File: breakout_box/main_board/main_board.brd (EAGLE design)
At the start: 60 x 120 mm, 31 parts, among them CN1 19PIN_LEMO, Q1 DMP3099L, Q2 DSS6060

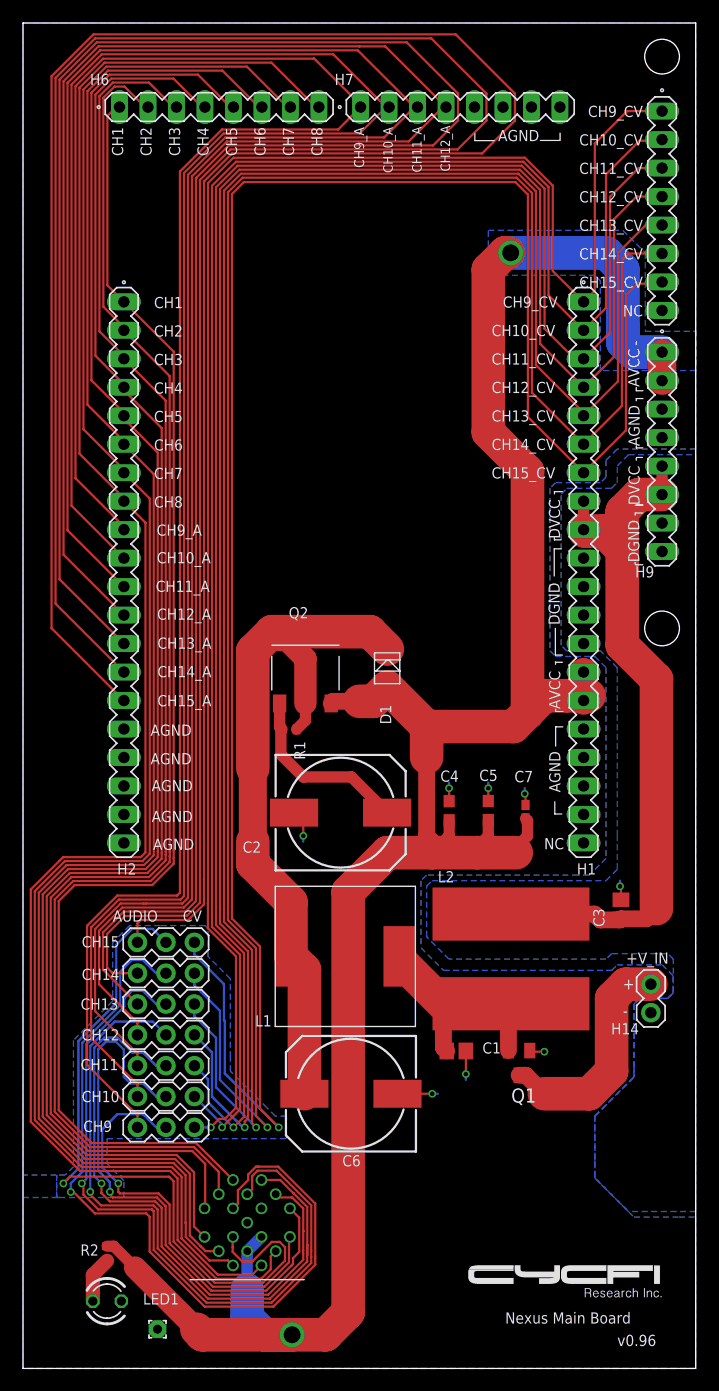
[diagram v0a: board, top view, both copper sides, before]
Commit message: commit and push eagle files for Nexus v2.3
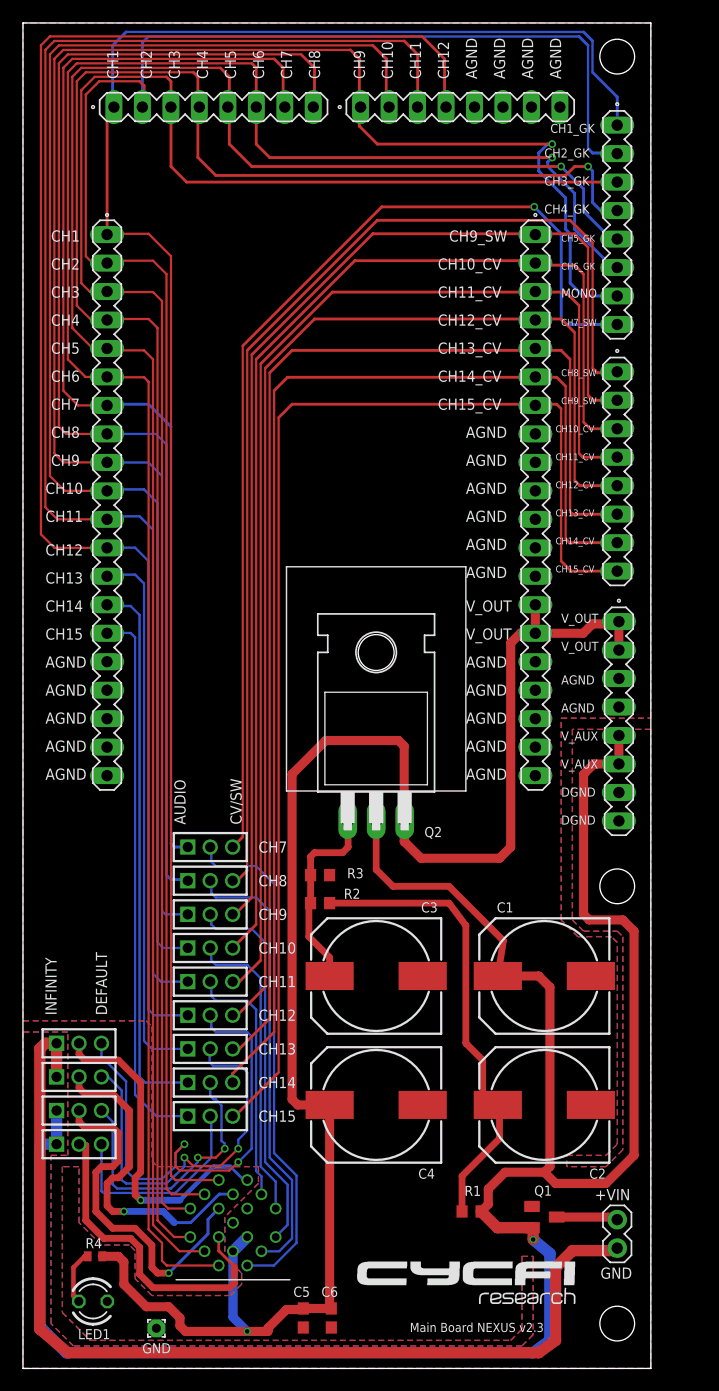
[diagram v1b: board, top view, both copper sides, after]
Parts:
- removed C7: 1nF, resistor:C0402K
- removed D1: FM4004W, CYCFI_diode:SMX
- removed H10, H11, H12, H13, H5: (no value), con-lstb:MA03-1_
- removed H14: MA02-1, con-lstb:MA02-1
- removed H9: (no value), con-lstb:MA08-1
- removed L1: 1mH, inductors:SDR
- removed L2: 82uH, resistor:L1280
- added H17: (no value), con-lstb:MA08-1
- added JP1, JP10, JP11, JP12, JP13, JP2, JP3, JP4, JP5, JP6, JP7, JP8, JP9: (no value), pinhead-2:1X03M
- added R3: 12k, resistor:R0603
- added R4: 4.7k, resistor:R0402
- C1, C3: value 22uF -> 470uF; device resistor:C0805 -> resistor:140CLH-1010
- C4: value 1uF -> 470uF; device resistor:C0603 -> resistor:140CLH-1010
- C5: value 10uF -> 1uF
- C6: value 1000uF -> 0.1uF; device resistor:140CLH-1010 -> resistor:C0603
- H1, H2: value (none) -> DNP
- H3, H4: device con-lstb:MA03-1_ -> con-lstb:MA08-1
- H6: value (none) -> MA02-1; device con-lstb:MA08-1 -> con-lstb:MA02-1
- Q2: value DSS6060 -> TIP122; device CYCFI_semicon:SOT-223-4 -> CYCFI_semicon:TO-220H
- R1: value 1k -> 220R; device resistor:R0402 -> resistor:R0603
- R2: value 4.7k -> 220R; device resistor:R0402 -> resistor:R0603
- moved H6 106.6 mm to (53.0, 12.0), turned to 90 degrees
- moved H4 81.6 mm to (39.0, 112.5)
- moved H3 80.1 mm to (17.0, 112.5)
- moved C5 48.2 mm to (25.0, 4.50), turned to 270 degrees
- moved R1 46.0 mm to (40.0, 14.0)
- moved H8 45.7 mm to (53.1, 57.7)
- moved R2 36.6 mm to (26.5, 41.5), turned to 0 degrees
- moved H7 35.4 mm to (53.0, 80.0), turned to 270 degrees
- moved C2 31.8 mm to (46.5, 23.5), turned to 180 degrees
- moved C4 27.0 mm to (31.5, 23.5), turned to 180 degrees
- moved C3 22.6 mm to (31.5, 35.0), turned to 180 degrees
- moved C6 20.1 mm to (27.5, 4.50), turned to 270 degrees
- moved Q1 13.9 mm to (46.5, 13.5), turned to 270 degrees
- moved C1 10.3 mm to (46.5, 35.0), turned to 180 degrees
- moved Q2 8.71 mm to (31.5, 56.5)
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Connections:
- removed net +AVCC: C4.1, C5.1, C7.1, CN1.P$16, CN1.P$17, D1.ANODE, H1.14, H1.15, H9.1, H9.2, Q2.P$3, R2.1
- removed net +DVCC: C3.1, H1.8, H1.9, H9.5, H9.6, L1.P$2
- removed net N$20: C2.+, Q2.P$1, R1.1
- new net GND1: H4.5, H4.6, H4.7, H4.8
- new net N$22: H2.15, JP9.1
- new net N$23: JP11.3, JP8.2
- new net N$31: CN1.P$3, H17.3, H2.3, H3.3
- new net N$39: CN1.P$4, H17.4, H2.4, H3.4
- new net N$40: JP12.3, JP7.2
- new net N$41: CN1.P$6, H17.6, H2.6, H3.6
- new net N$43: H2.8, H3.8, JP2.1
- new net N$44: JP13.3, JP6.2
- new net V_AUX: C1.+, H8.5, H8.6, JP10.1, JP11.1, Q1.2, Q2.2, R1.2
- new net V_OUT: C4.+, C5.1, C6.1, CN1.P$16, CN1.P$17, H1.12, H1.13, H1.14, H1.15, H8.1, H8.2, Q2.3, R4.1
- net GND: now also C1.-, C3.-, C4.-, C6.2, H1.8, H1.9, H6.1, H8.3, H8.4, H8.7, H8.8, JP12.1, JP13.1, R3.1; no longer C1.2, C3.2, C4.2, C6.-, C7.2, H1.12, H1.13, H14.1, H7.5, H7.6, H7.7, H7.8, H9.3, H9.4, H9.7, H9.8
- net N$1: now also CN1.P$2, H17.2, H2.2, H3.2; no longer H2.13, H3.1
- net N$10: now also JP10.3, JP9.2; no longer CN1.P$6, H2.6, H6.6
- net N$11: now also H3.7, JP1.1; no longer CN1.P$7, H6.7
- net N$12: now also CN1.P$7, JP1.2; no longer CN1.P$8, H2.8, H6.8
- net N$13: now also H1.1, H7.2, JP3.3; no longer CN1.P$9, H10.2
- net N$14: now also JP4.2; no longer H11.2
- net N$15: now also JP5.2; no longer H12.2
- net N$16: now also JP13.2; no longer H13.2
- net N$17: now also CN1.P$9, JP3.2; no longer H2.15, H5.1
- net N$18: now also H4.2, JP4.1; no longer H11.1, H7.2
- net N$19: now also H2.13, JP7.1; no longer C1.1, L1.P$1, L2.P$1, Q1.2
- net N$2: now also CN1.P$1, H17.1, H2.1, H3.1; no longer H14.2, Q1.3
- net N$21: now also H2.14, JP8.1; no longer C6.+, D1.CATHODE, L2.P$2, Q2.P$2, Q2.P$4, R1.2
- net N$25: now also R4.2; no longer R2.2
- net N$26: now also H7.4, JP5.3; no longer H12.3, H8.3
- net N$27: now also H7.3, JP4.3; no longer H11.3, H8.2
- net N$28: now also H4.4, JP6.1; no longer H13.1, H7.4
- net N$29: now also H4.3, JP5.1; no longer H12.1, H7.3
- net N$3: now also CN1.P$8, JP2.2; no longer H2.14, H4.1
- net N$30: now also H7.5, JP6.3; no longer H13.3, H8.4
- net N$32: now also H17.7, H4.1, JP3.1; no longer H10.1, H7.1
- net N$33: now also H7.6, JP7.3; no longer H3.3, H8.5
- net N$34: now also H7.7, JP8.3; no longer H4.3, H8.6
- net N$35: now also H7.8, JP9.3; no longer H5.3, H8.7
- net N$36: now also JP12.2; no longer H3.2
- net N$37: now also JP11.2; no longer H4.2
- net N$38: now also JP10.2; no longer H5.2
- net N$4: now also H6.2, Q1.3; no longer CN1.P$1, H2.1, H6.1
- net N$5: now also H7.1, JP2.3; no longer CN1.P$2, H2.2, H6.2
- net N$6: now also C3.+, Q2.1, R2.1, R3.2; no longer CN1.P$3, H2.3, H6.3
- net N$7: now also H17.8, JP1.3; no longer CN1.P$4, H2.4, H6.4
- net N$8: now also C2.+, R1.1, R2.2; no longer CN1.P$5, H2.5, H6.5
- net N$9: now also CN1.P$5, H17.5, H2.5, H3.5; no longer H1.1, H10.3, H8.1
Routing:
- net +AVCC: track 222.3 -> 0.00 mm, vias 2 -> 0
- net V_AUX: track 0.00 -> 187.7 mm, vias 0 -> 1
- net N$41: track 0.00 -> 182.5 mm, vias 0 -> 1
- net N$17: track 208.6 -> 34.0 mm
- net N$39: track 0.00 -> 172.2 mm, vias 0 -> 1
- net N$3: track 207.4 -> 40.2 mm
- net N$31: track 0.00 -> 165.8 mm
- net V_OUT: track 0.00 -> 153.9 mm, vias 0 -> 1
- net N$2: track 20.3 -> 162.4 mm
- net N$10: track 147.0 -> 19.1 mm
- net N$12: track 159.5 -> 45.8 mm
- net N$4: track 119.1 -> 5.50 mm
- net N$6: track 129.4 -> 17.6 mm
- net N$43: track 0.00 -> 110.3 mm
- net N$8: track 140.5 -> 42.7 mm
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- added copper zone on layer 1, net GND
- removed copper zone on layer 16, net N$22
- removed copper zone on layer 16, net N$23
- removed copper zone on layer 16, net N$24
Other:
- board size 60 x 120 mm -> 56 x 120 mm
- board text added: "+VIN"
- board text added: "CH1_GK"
- board text added: "CH2_GK"
- board text added: "CH3_GK"
- board text added: "CH4_GK"
- board text added: "CH5_GK"
- board text added: "CH6_GK"
- board text added: "CH7_SW"
- board text added: "CH8_SW"
- board text added: "CH9_SW"
- board text added: "CV/SW"
- board text added: "DEFAULT"
- board text added: "GND"
- board text added: "INFINITY"
- board text added: "MONO"
- board text added: "Main Board NEXUS v2.3"
- board text added: "V_AUX"
- board text added: "V_OUT"
- board text removed: "+"
- board text removed: "+V_IN"
- board text removed: "-"
- board text removed: "AVCC"
- board text removed: "CH10_A"
- board text removed: "CH11_A"
- board text removed: "CH12_A"
- board text removed: "CH13_A"
- board text removed: "CH14_A"
- board text removed: "CH15_A"
- board text removed: "CH9_A"
- board text removed: "CH9_CV"
- board text removed: "CV"
- board text removed: "DVCC"
- board text removed: "H14"
- board text removed: "L1"
- board text removed: "L2"
- board text removed: "NC"
- board text removed: "Nexus Main Board"
- board text removed: "Q2"
- board text removed: "v0.96"

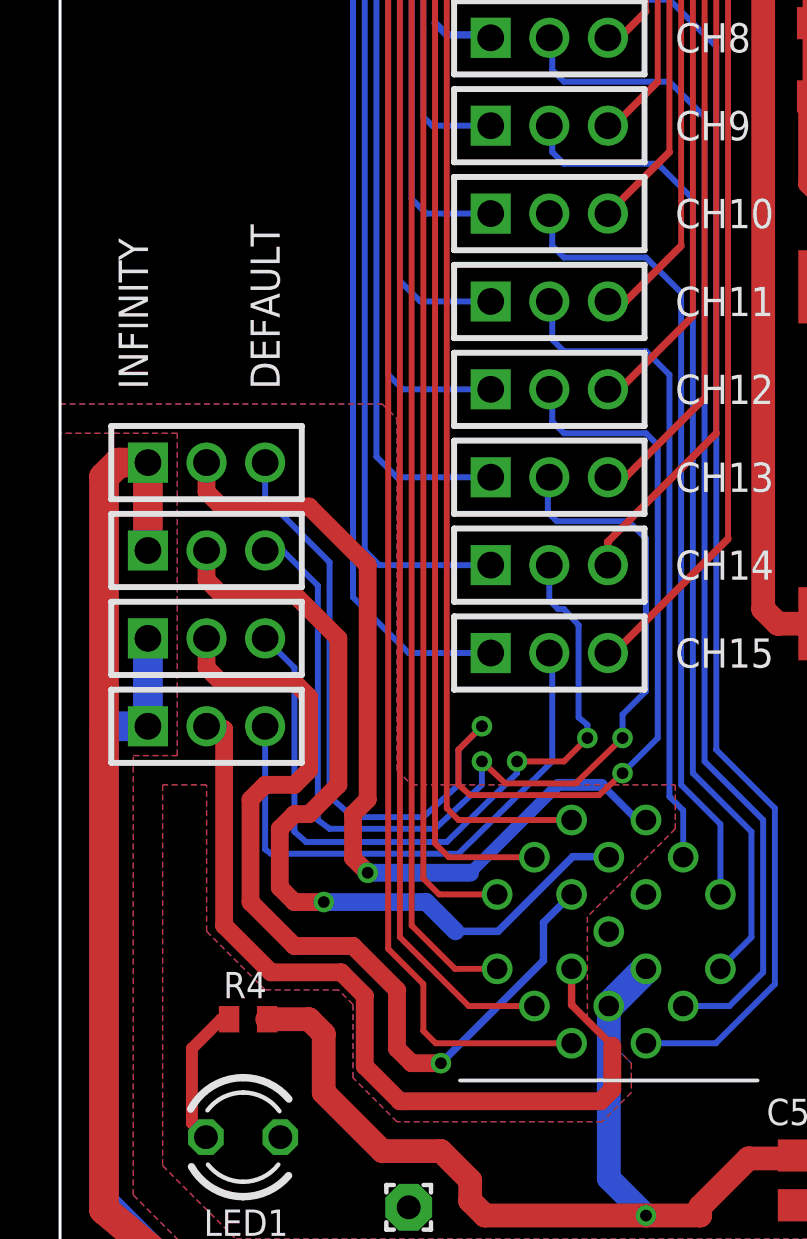
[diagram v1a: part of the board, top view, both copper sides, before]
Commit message: Updates in Mainboard
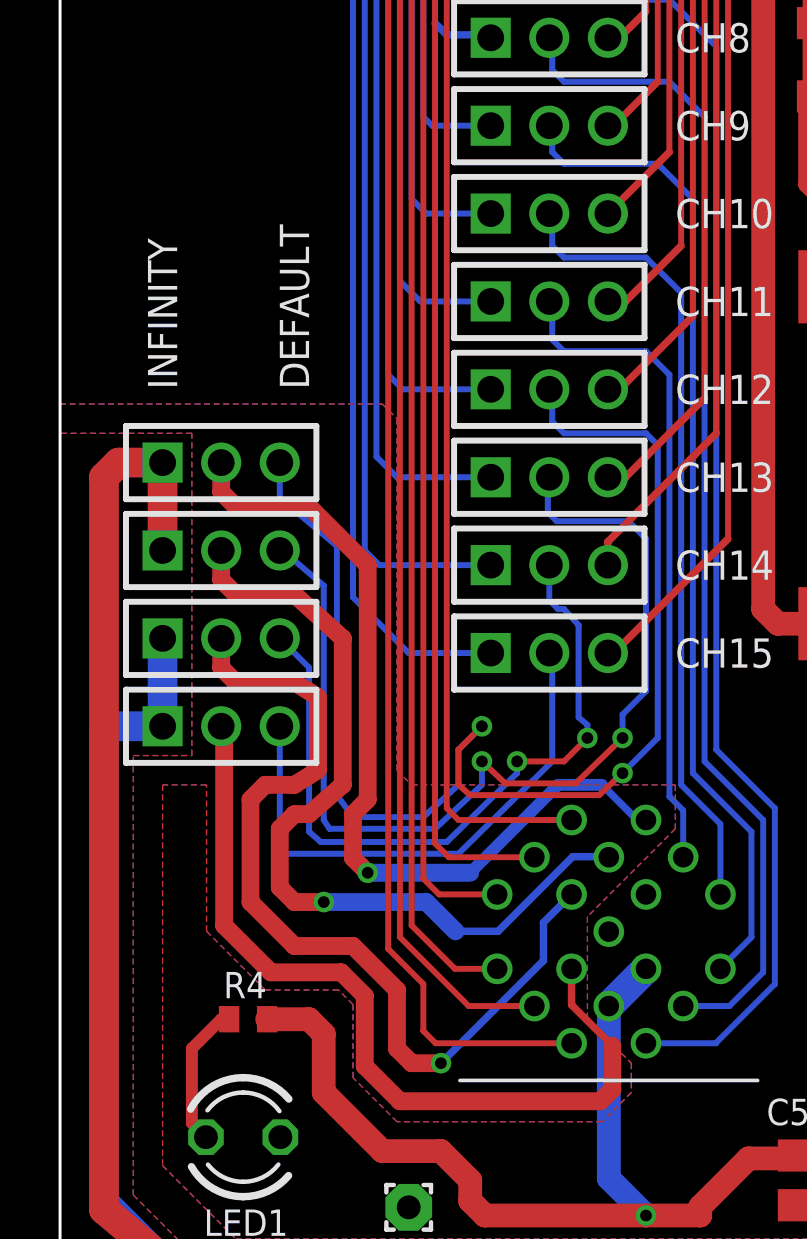
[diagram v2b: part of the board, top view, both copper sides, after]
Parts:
- moved JP10 0.50 mm to (5.50, 20.0)
- moved JP11 0.50 mm to (5.50, 23.0)
- moved JP12 0.50 mm to (5.50, 26.0)
- moved JP13 0.50 mm to (5.50, 29.0)
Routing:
- net N$23: track 25.4 -> 24.9 mm
- net V_AUX: track 187.7 -> 188.2 mm
- net N$16: track 29.7 -> 29.2 mm
- net N$10: track 19.1 -> 18.6 mm
- net GND: track 89.5 -> 90.0 mm

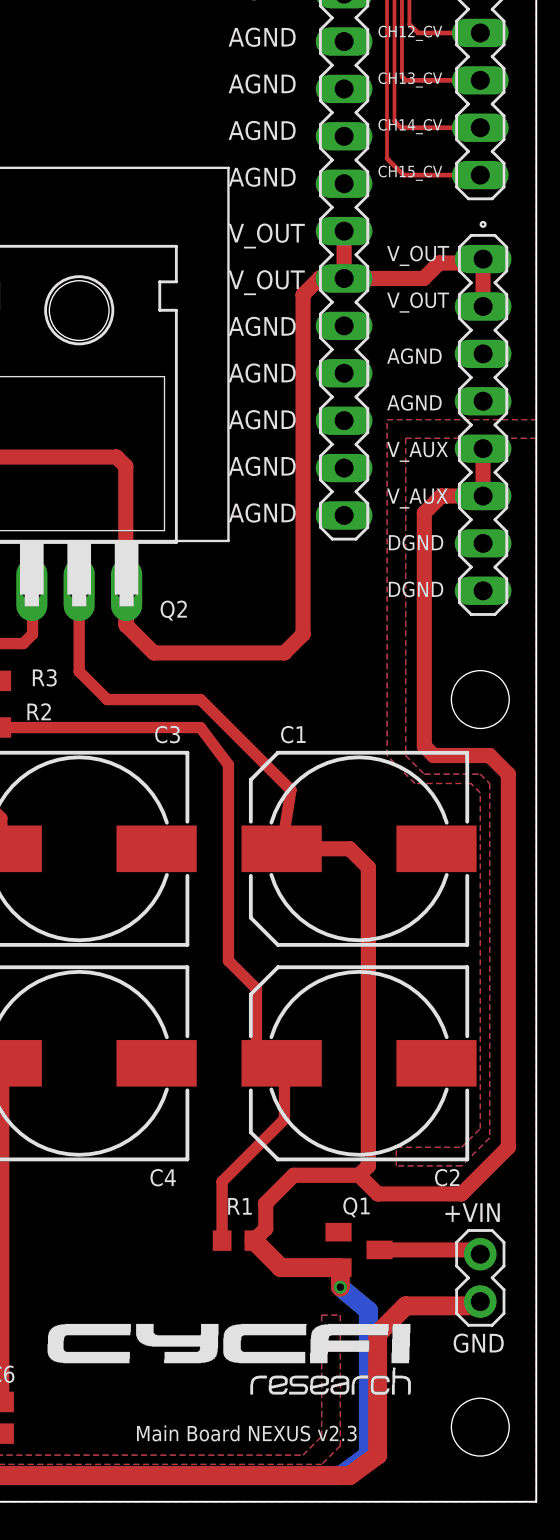
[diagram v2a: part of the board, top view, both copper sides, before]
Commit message: updates
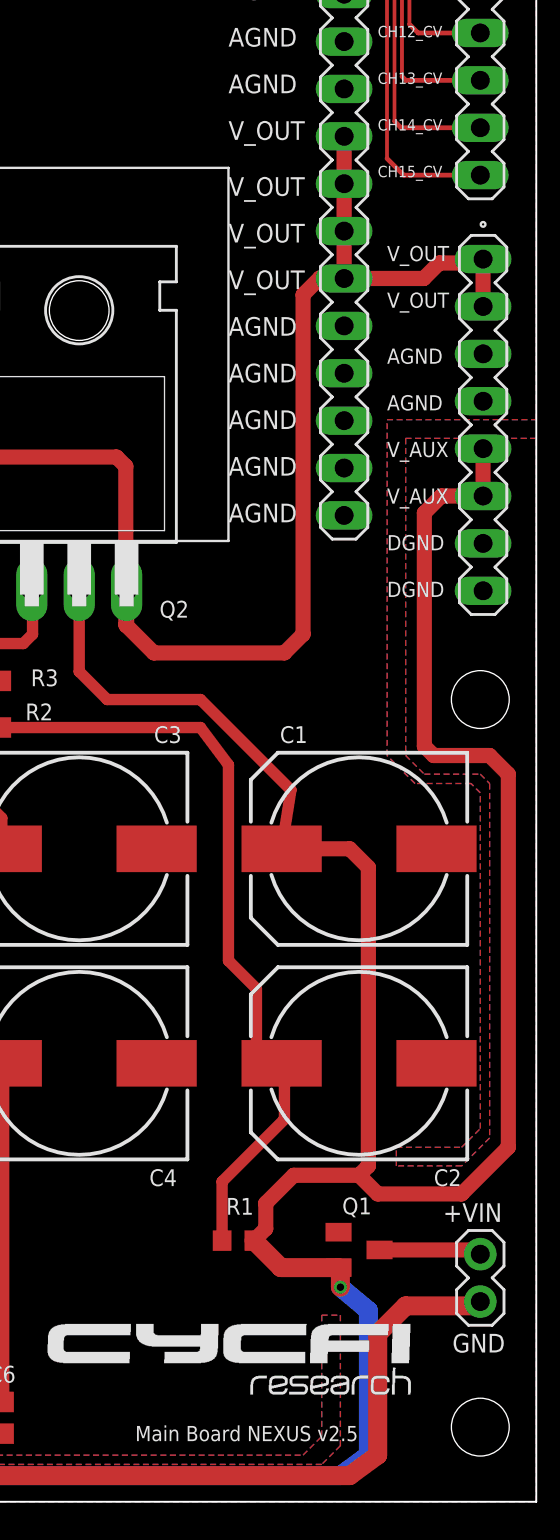
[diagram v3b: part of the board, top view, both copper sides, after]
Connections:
- removed net GND1: H4.5, H4.6, H4.7, H4.8
- net GND: now also H1.20, H4.5, H4.6, H4.7, H4.8
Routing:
- net V_OUT: track 153.9 -> 158.9 mm
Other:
- board text added: "Main Board NEXUS v2.5"
- board text removed: "Main Board NEXUS v2.3"
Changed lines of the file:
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@@
 <rectangle x1="44.8369" y1="9.5077" x2="48.0881" y2="9.5331" layer="25"/>
 <rectangle x1="48.3167" y1="9.5077" x2="49.2565" y2="9.5331" layer="25"/>
-<text x="34.5" y="3.25" size="0.8128" layer="25" font="vector" ratio="12">Main Board NEXUS v2.3</text>
+<text x="34.5" y="3.25" size="0.8128" layer="25" font="vector" ratio="12">Main Board NEXUS v2.5</text>
 <text x="2.5" y="100.5" size="1" layer="25" font="vector" ratio="12">CH1</text>
 <text x="2.5" y="98" size="1" layer="25" font="vector" ratio="12">CH2</text>
@@
 <text x="39.5" y="78" size="1" layer="25" font="vector" ratio="12">AGND</text>
 <text x="39.5" y="75.5" size="1" layer="25" font="vector" ratio="12">AGND</text>
-<text x="39.5" y="73" size="1" layer="25" font="vector" ratio="12">AGND</text>
-<text x="39.5" y="70.5" size="1" layer="25" font="vector" ratio="12">AGND</text>
 <text x="39.5" y="62.5" size="1" layer="25" font="vector" ratio="12">AGND</text>
 <text x="39.5" y="60" size="1" layer="25" font="vector" ratio="12">AGND</text>
@@
 <text x="48" y="115" size="1" layer="25" font="vector" ratio="12" rot="R90">AGND</text>
 <hole x="31.5" y="63.85" drill="3.2"/>
+<text x="39.5" y="70" size="1" layer="25" font="vector" ratio="12">V_OUT</text>
+<text x="39.5" y="73" size="1" layer="25" font="vector" ratio="12">V_OUT</text>
 </plain>
 <attributes>
@@
 <vertex x="56" y="0"/>
 </polygon>
+<contactref element="H1" pad="20"/>
+<contactref element="H4" pad="5"/>
+<contactref element="H4" pad="6"/>
+<contactref element="H4" pad="7"/>
+<contactref element="H4" pad="8"/>
 </signal>
 <signal name="N$14">
@@
 <wire x1="23.5" y1="5.25" x2="24.9" y2="5.25" width="0.8128" layer="1"/>
 <wire x1="24.9" y1="5.25" x2="25" y2="5.35" width="0.8128" layer="1"/>
-<wire x1="45.7" y1="70.65" x2="45.7" y2="73.19" width="0" layer="19" extent="1-1"/>
-<wire x1="45.7" y1="68.11" x2="45.7" y2="70.65" width="0" layer="19" extent="1-1"/>
+<wire x1="45.7" y1="68.11" x2="45.7" y2="70.65" width="0.8128" layer="1"/>
+<wire x1="45.7" y1="70.65" x2="45.7" y2="73.19" width="0.8128" layer="1"/>
 </signal>
 <signal name="N$31">
@@
 <wire x1="41.35" y1="23" x2="41" y2="23" width="0.4064" layer="1"/>
 </signal>
-<signal name="GND1">
-<contactref element="H4" pad="5"/>
-<contactref element="H4" pad="6"/>
-<contactref element="H4" pad="7"/>
-<contactref element="H4" pad="8"/>
-<wire x1="45.35" y1="112.5" x2="47.89" y2="112.5" width="0" layer="19" extent="1-1"/>
-<wire x1="42.81" y1="112.5" x2="45.35" y2="112.5" width="0" layer="19" extent="1-1"/>
-<wire x1="40.27" y1="112.5" x2="42.81" y2="112.5" width="0" layer="19" extent="1-1"/>
-</signal>
 <signal name="N$2">
